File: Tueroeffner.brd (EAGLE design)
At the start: 54.6 x 22.9 mm, 34 parts, among them IC1 NCP1117ST33T3G, IC3 M25PE20, K1 EC2-12SNU, Q1 2N7002CK, Q3 2N7002CK

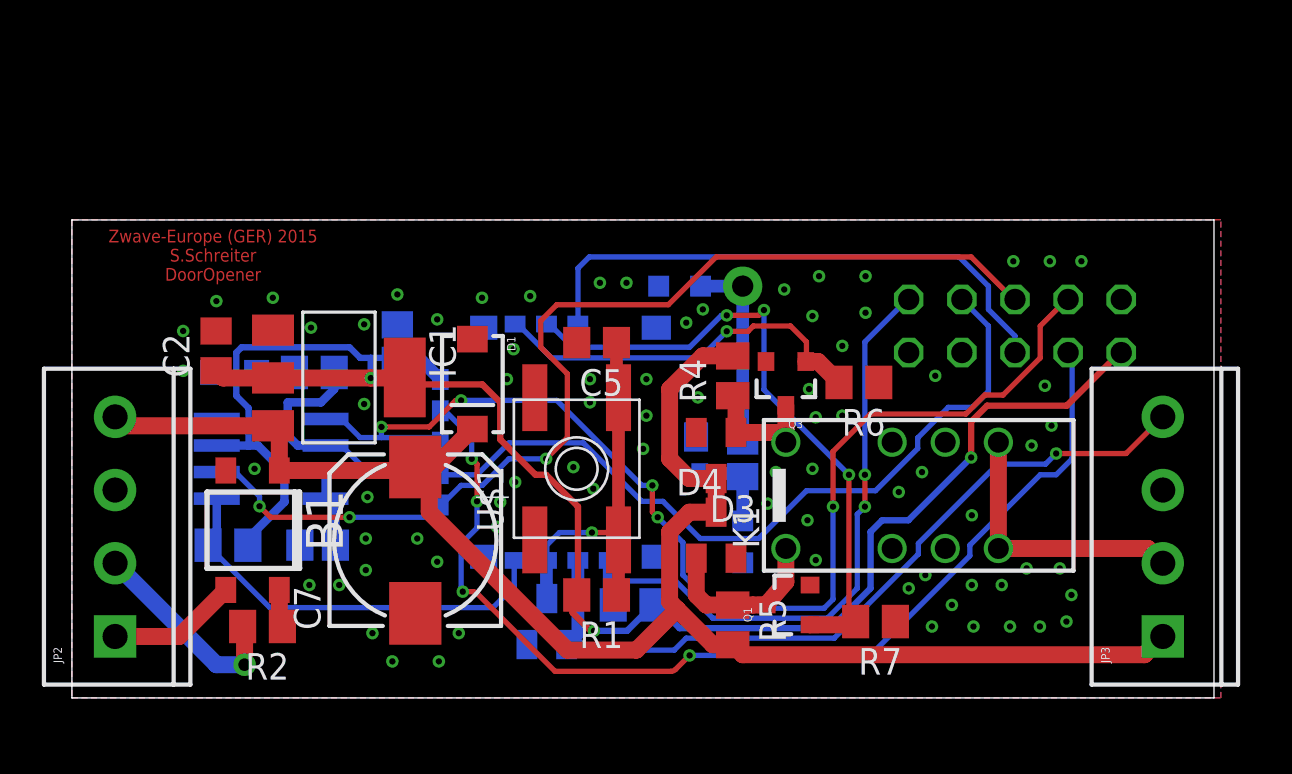
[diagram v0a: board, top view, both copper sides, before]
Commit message: New H-Bridge
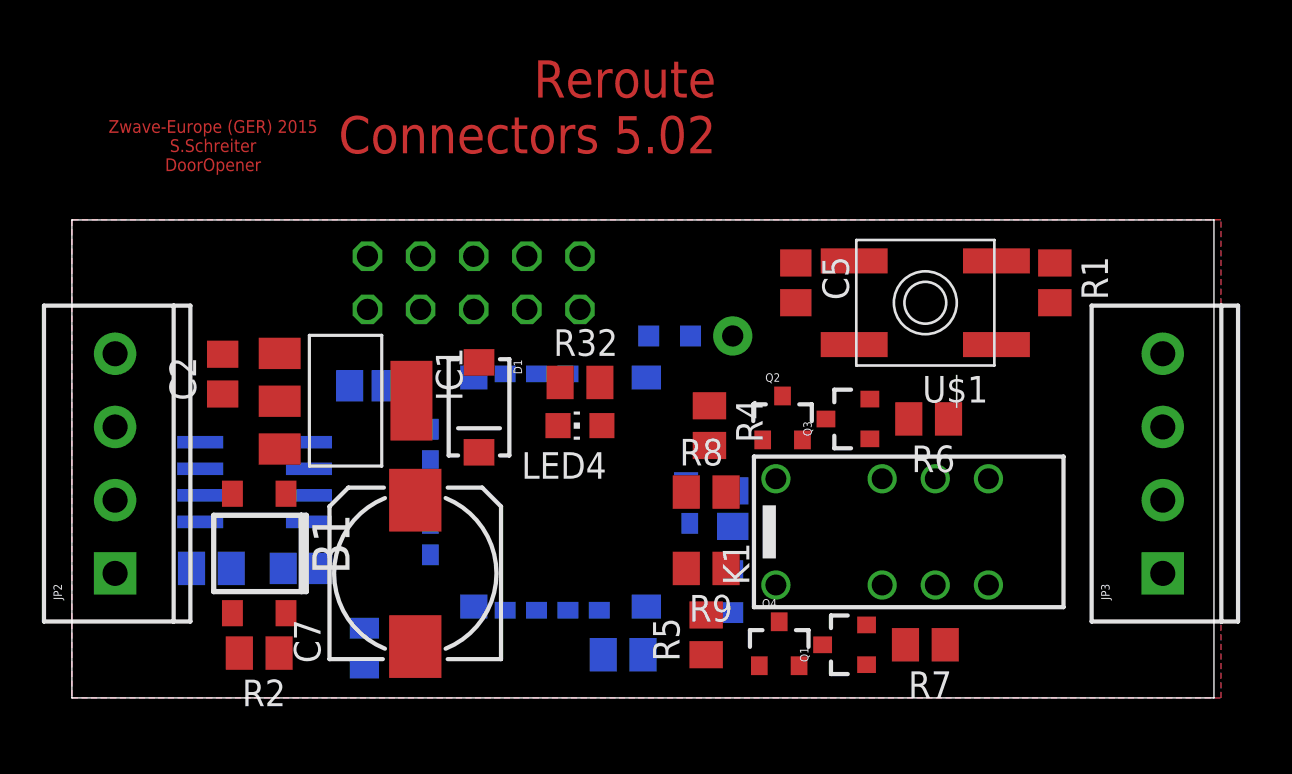
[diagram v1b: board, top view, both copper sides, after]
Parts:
- removed D3, D4: PMBD914, semicon-smd-ipc:SOT23
- added Q2, Q4: 2N7002CK, SparkFun-DiscreteSemi:SOT23-3
- added R8, R9: 100, resistor:M2012
- R4, R5: value 47 -> 10K
- moved R1 26.5 mm to (45.4, 18.6), turned to 270 degrees
- moved SV3 26.0 mm to (17.6, 18.6), turned to 180 degrees
- moved U$1 18.5 mm to (39.2, 17.6), turned to 180 degrees
- moved LED4 16.7 mm to (22.7, 11.7), flipped to the top, turned to 90 degrees
- moved R32 12.7 mm to (22.7, 13.8), flipped to the top
- moved C5 9.94 mm to (33.0, 18.6), turned to 270 degrees
- moved D2 7.73 mm to (13.5, 1.11), turned to 90 degrees
- moved R6 3.76 mm to (39.4, 12.1)
- moved Q3 3.49 mm to (35.6, 12.1), turned to 90 degrees
- moved Q1 3.30 mm to (35.4, 1.27)
- moved JP2 3.02 mm to (0.48, 4.68)
- moved JP3 3.02 mm to (50.6, 4.68)
- moved R7 2.63 mm to (39.2, 1.27)
- moved R4 2.63 mm to (28.9, 11.7), turned to 270 degrees
- moved C3 2.51 mm to (12.5, 13.7), turned to 0 degrees
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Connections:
- new net N$4: R8.2, U$5.14
- new net N$5: R9.2, U$5.13
- net DC_5-12V: now also Q2.3, Q4.3; no longer D3.3, D4.3, R4.2, R5.2
- net GND: now also R4.1, R5.1
- net N$2: now also Q2.2; no longer D3.1, R4.1
- net N$3: now also Q4.2; no longer D4.1, R5.1
- net RELAY0: now also Q2.1, R4.2, R8.1; no longer U$5.14
- net RELAY1: now also Q4.1, R5.2, R9.1; no longer U$5.13
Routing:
- net VCC-3.3V: track 92.0 -> 0.00 mm, vias 3 -> 0
- net DC_5-12V: track 80.1 -> 0.00 mm
- net MOSI: track 56.8 -> 0.00 mm, vias 5 -> 0
- net MISO: track 50.4 -> 0.00 mm, vias 3 -> 0
- net RXD: track 50.3 -> 0.00 mm, vias 4 -> 0
- net SCK: track 49.9 -> 0.00 mm
- net INT1: track 37.5 -> 0.00 mm, vias 1 -> 0
- net RELAY0: track 30.7 -> 0.00 mm, vias 3 -> 0
- net RESET: track 30.3 -> 0.00 mm, vias 2 -> 0
- net TXD: track 26.8 -> 0.00 mm
- net CS: track 19.9 -> 0.00 mm
- net BUTTON: track 19.2 -> 0.00 mm, vias 1 -> 0
- net RELAY1: track 18.5 -> 0.00 mm, vias 1 -> 0
- net RELAY: track 13.2 -> 0.00 mm
- net AC_5-12V0: track 10.0 -> 0.00 mm, vias 1 -> 0
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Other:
- board text added: "Reroute Connectors 5.02"

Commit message: Basic Routing
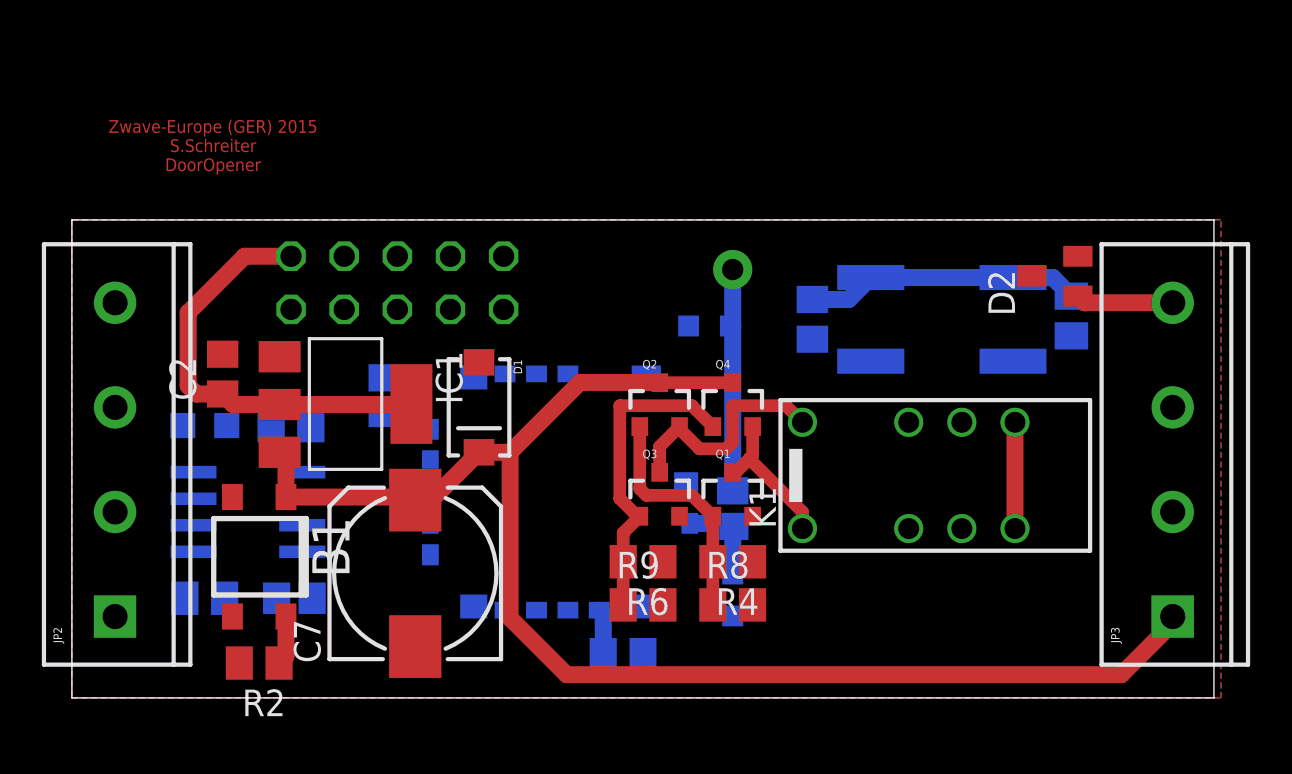
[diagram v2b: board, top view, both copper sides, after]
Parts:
- removed R5, R7: 10K, resistor:M2012
- moved D2 36.5 mm to (45.4, 18.9), flipped to the top
- moved LED4 17.9 mm to (4.76, 11.7), flipped to the bottom, turned to 270 degrees
- moved R6 15.3 mm to (25.7, 5.24)
- moved R32 14.0 mm to (8.89, 11.7), flipped to the bottom
- moved Q4 11.6 mm to (30.0, 12.7)
- moved Q3 9.76 mm to (26.5, 8.41), turned to 0 degrees
- moved Q1 8.95 mm to (30.0, 8.41), turned to 0 degrees
- moved R4 6.60 mm to (30.0, 5.24), turned to 180 degrees
- moved Q2 5.91 mm to (26.5, 12.7)
- moved R8 5.54 mm to (30.0, 3.17)
- moved SV3 3.65 mm to (14.0, 18.6)
- moved R9 3.49 mm to (25.7, 3.17), turned to 0 degrees
- moved JP1 3.17 mm to (30.0, 19.2)
- moved K1 2.98 mm to (39.7, 9.37)
- moved JP3 2.12 mm to (51.0, 2.62)
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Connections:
- net GND: no longer R5.1, R7.1
- net RELAY0: no longer R7.2
- net RELAY1: no longer R5.2
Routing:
- net DC_5-12V: track 0.00 -> 68.1 mm
- net VCC-3.3V: track 0.00 -> 23.1 mm
- net RELAY1: track 0.00 -> 15.2 mm
- net BUTTON: track 0.00 -> 13.2 mm
- net RELAY0: track 0.00 -> 11.2 mm
- net N$2: track 0.00 -> 11.2 mm
- net N$33: track 0.00 -> 10.7 mm
- net N$3: track 0.00 -> 7.05 mm
- net RELAY: track 0.00 -> 5.08 mm
- net INT1: track 0.00 -> 4.67 mm
- net ANTENNA: track 0.00 -> 4.48 mm
- net N$1: track 0.00 -> 2.36 mm
- net RESET: track 0.00 -> 2.21 mm
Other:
- board text removed: "Reroute Connectors 5.02"
